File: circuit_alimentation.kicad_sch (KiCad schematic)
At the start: 31 parts, among them U1 STM32-(STM32H745ZIT6)

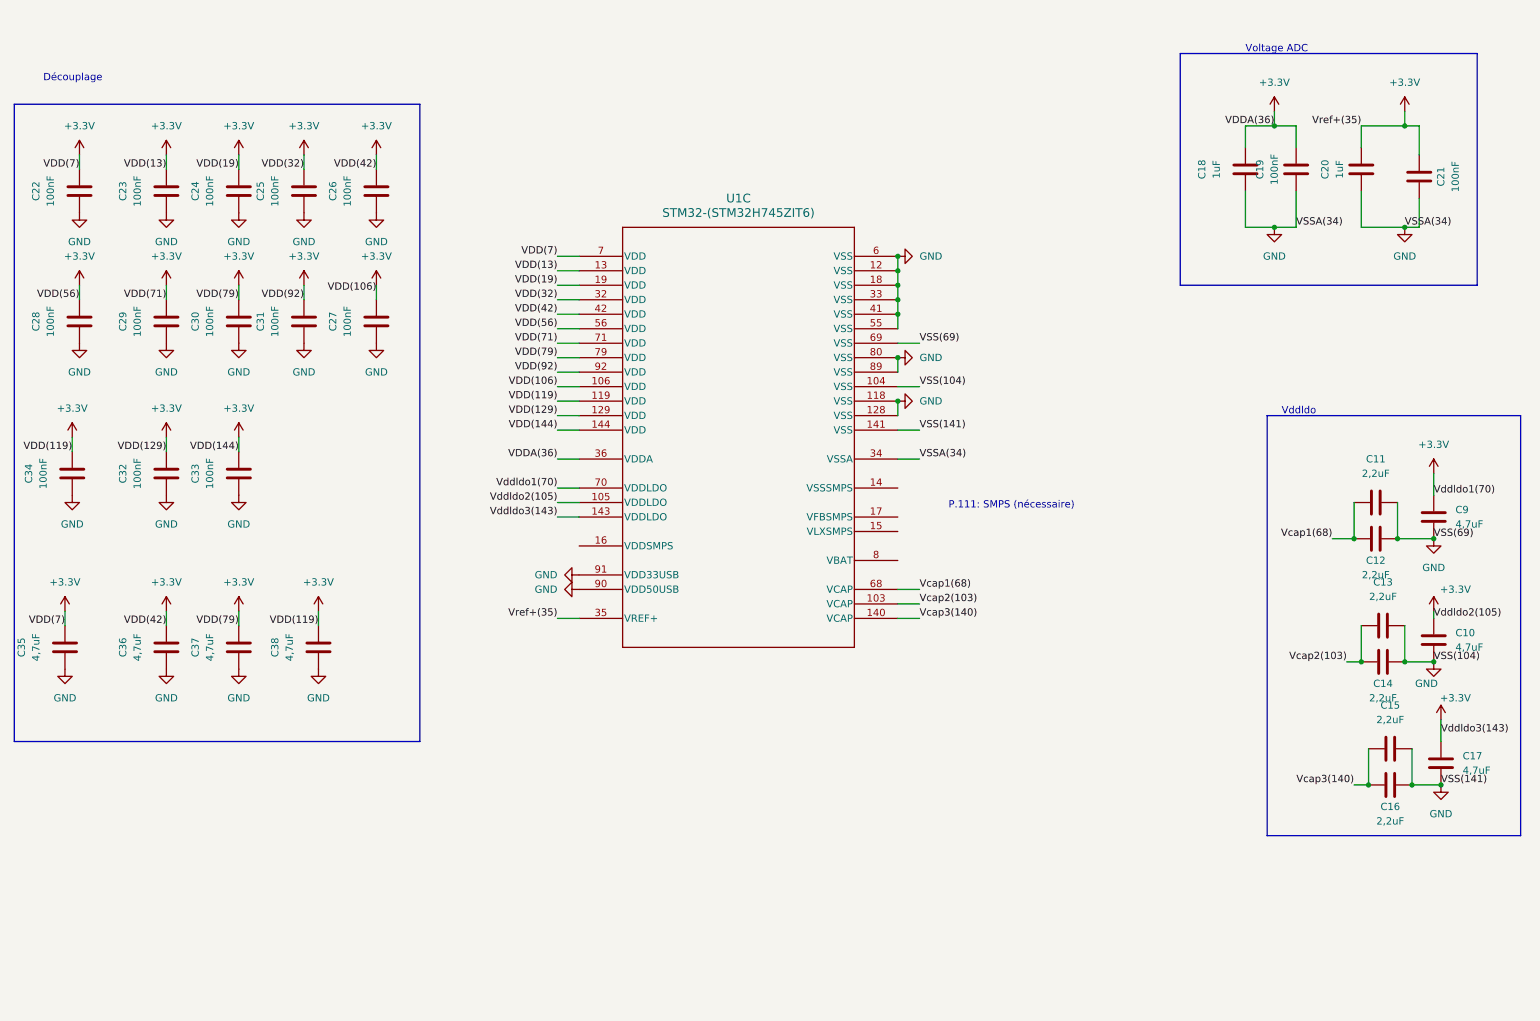
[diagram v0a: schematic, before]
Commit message: Revert "Recommit du Vbuck"
This reverts commit db6b1385e92bec759ec8c6f30127fdc08b8b4918.
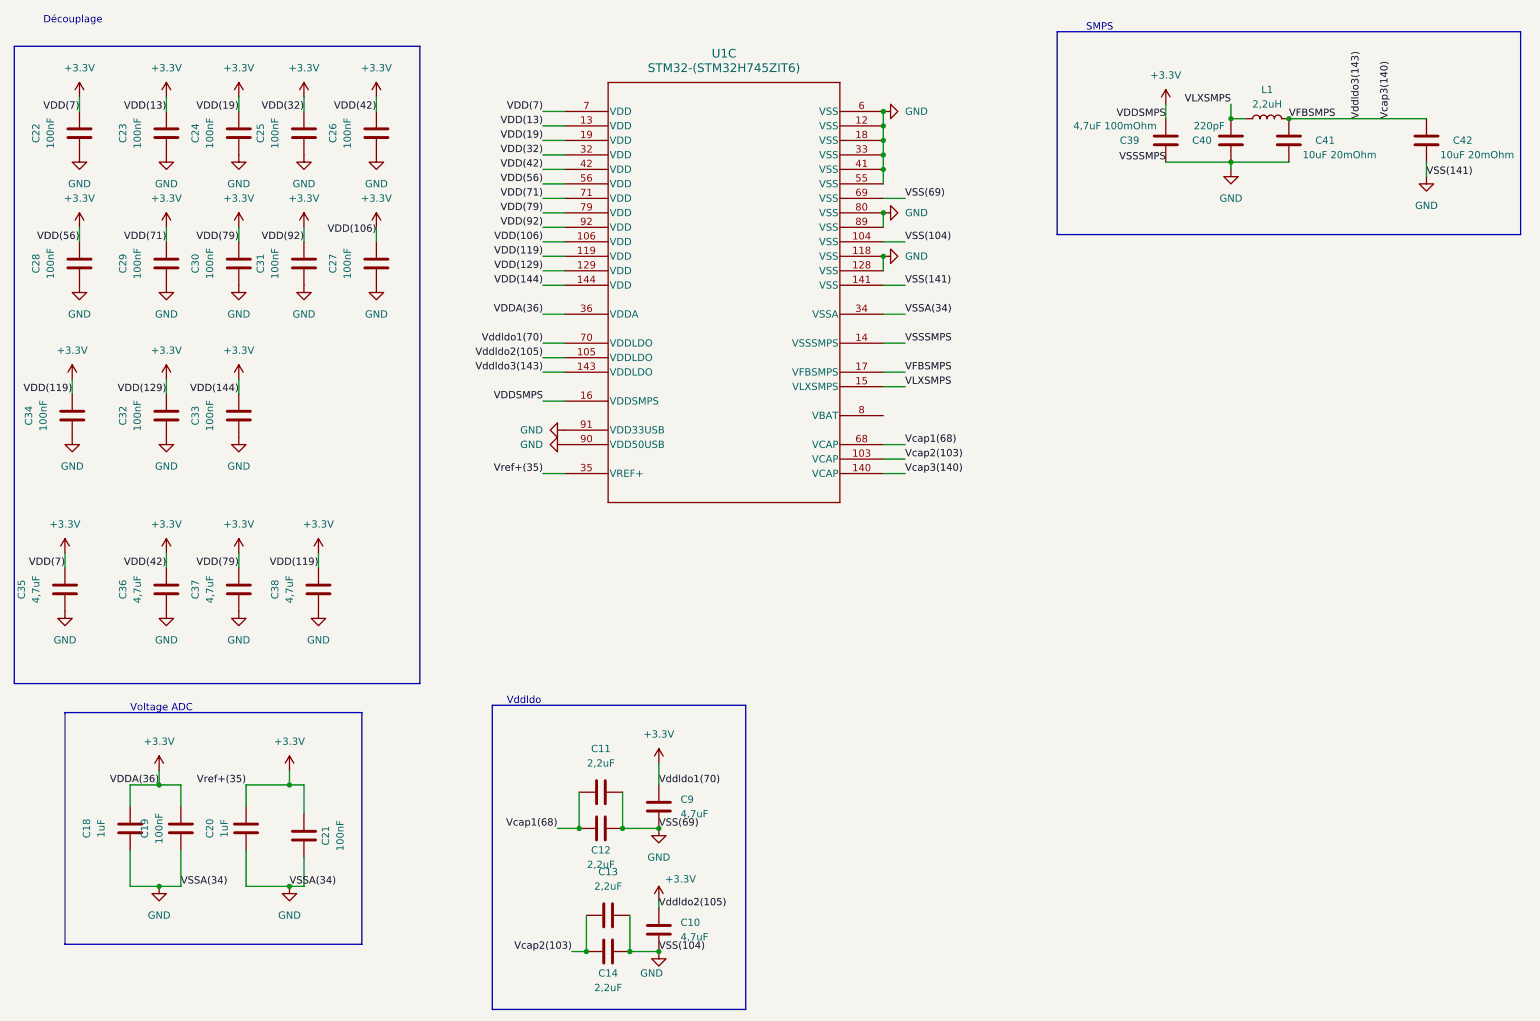
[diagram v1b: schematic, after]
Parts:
- removed C15, C16: 2,2uF, symbol Device:C
- removed C17: 4,7uF, symbol Device:C
- added C39: 4,7uF 100mOhm, symbol Device:C
- added C40: 220pF, symbol Device:C
- added C41, C42: 10uF 20mOhm, symbol Device:C
- added L1: 2,2uH, symbol Device:L
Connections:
- net Vcap3(140) is gone; now on net VFBSMPS: U1.140 (VCAP)
- net +3.3V: now also U1.16 (VDDSMPS), C39.1; no longer U1.143 (VDDLDO)
- net GND: now also U1.14 (VSSSMPS), C39.2, C40.2, C41.1, C42.1
- net VLXSMPS: now reaches U1.15 (VLXSMPS)
- net VLXSMPS: now also C40.1, L1.1
- net VFBSMPS: now reaches U1.17 (VFBSMPS)
- net VFBSMPS: now also U1.143 (VDDLDO), C41.2, C42.2, L1.2
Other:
- note added: "SMPS"
- note removed: "P.111: SMPS (nécessaire)"
- moved on the sheet: C10, C11, C12, C13, C14, C18, C19, C20, C21, C22, C23, C24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
